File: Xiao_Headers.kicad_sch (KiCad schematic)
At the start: 28 parts, among them J1 Barrel_Jack, P1 USB_C_Plug_USB2.0, SW1 SW_Push, SW2 SW_Push, U1 SHT4x, U2 ESP32-C3-WROOM-02, U3 TSL25911FN, U5 LT1963AxST-3.3

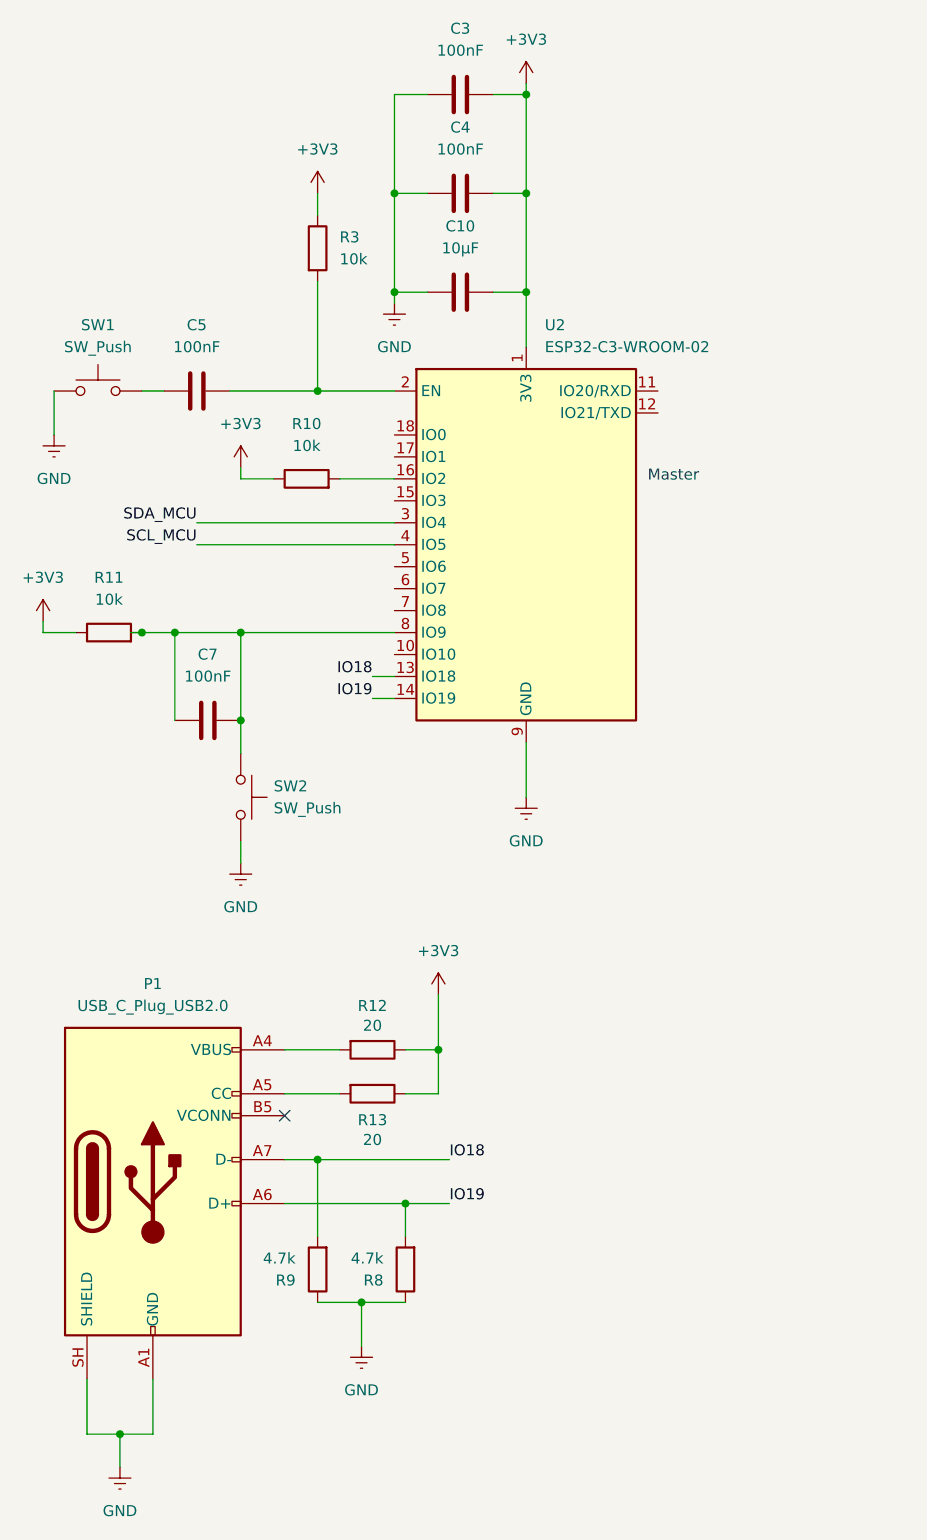
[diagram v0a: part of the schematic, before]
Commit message: Schematics Confirmed
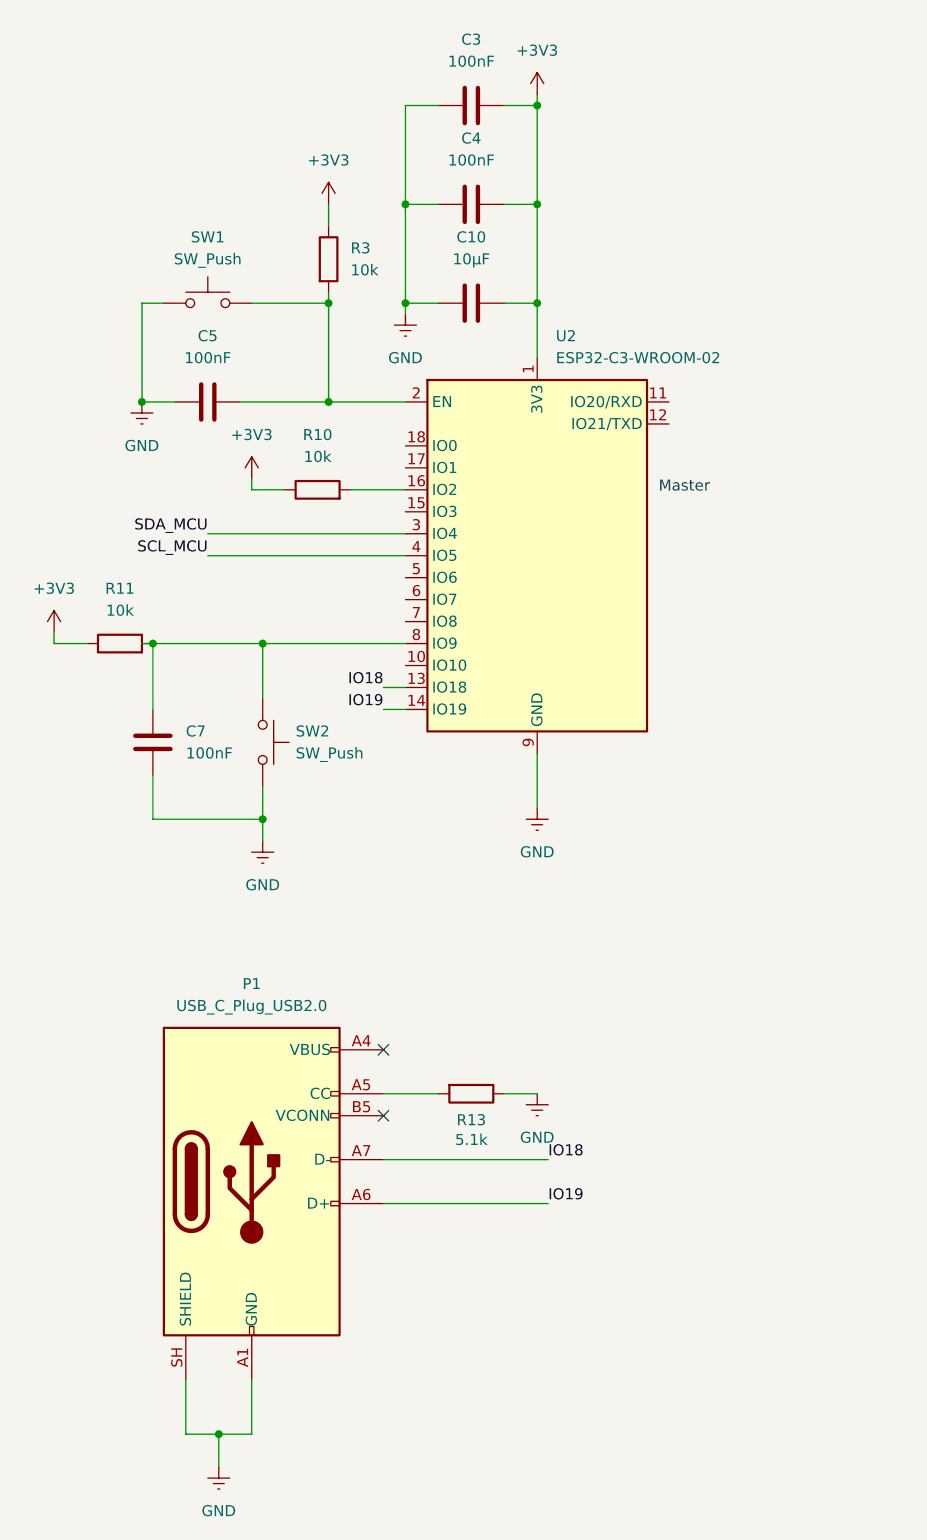
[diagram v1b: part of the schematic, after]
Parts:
- removed R12: 20, symbol Device:R
- removed R8, R9: 4.7k, symbol Device:R
- R13: value 20 -> 5.1k
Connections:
- net +3V3: now also C5.1, C7.2
- net at SW1.2: now also C5.2, R3.2, U2.2 (EN); no longer C5.1
- net at C7.1, R11.2, SW2.1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: no longer C7.2
- no-connect marks 2 -> 3
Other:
- moved on the sheet: C10, C3, C4, C5, C7, P1, R10, R11, R13, R3, SW1, SW2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
